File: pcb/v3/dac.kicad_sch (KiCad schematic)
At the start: 64 parts, among them U14 CS43198, U15 CS43198, U16 OPA1622

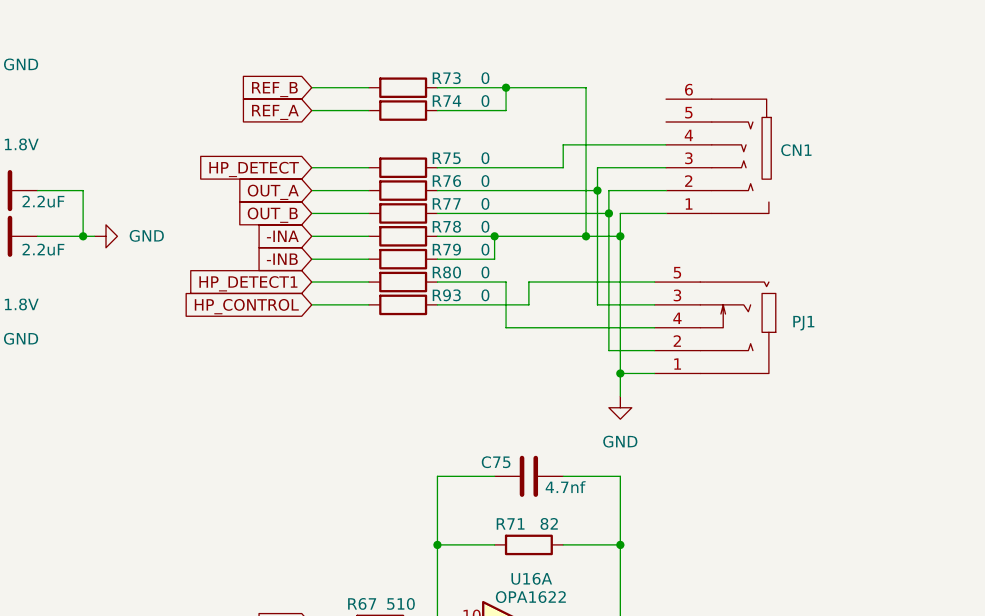
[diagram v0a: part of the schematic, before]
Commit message: up
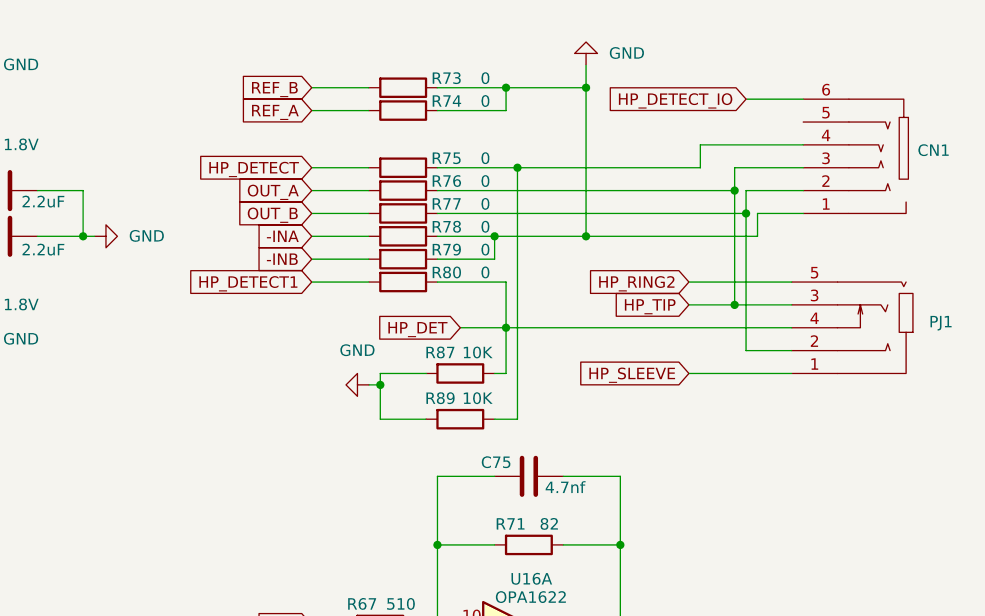
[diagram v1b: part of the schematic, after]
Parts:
- removed R93: 0, Resistor_SMD:R_0805_2012Metric, symbol Device:R
- added R87, R89: 10K, Capacitor_SMD:C_0402_1005Metric_Pad0.74x0.62mm_HandSolder, symbol Device:R
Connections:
- net GND: now also R87.2, R89.2; no longer PJ1.1
- net HP_TIP: now reaches CN1.3, PJ1.3, R76.1
- net HP_DET: now reaches PJ1.4, R80.1
- net HP_DET: now also R87.1
- net HP_RING2: now reaches PJ1.5
- net at CN1.4 (3), R75.1: now also R89.1
- net HP_DETECT_IO: now reaches CN1.6
- new net HP_SLEEVE: PJ1.1
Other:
- moved on the sheet: CN1, PJ1
